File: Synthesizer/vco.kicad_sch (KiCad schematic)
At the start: 33 parts

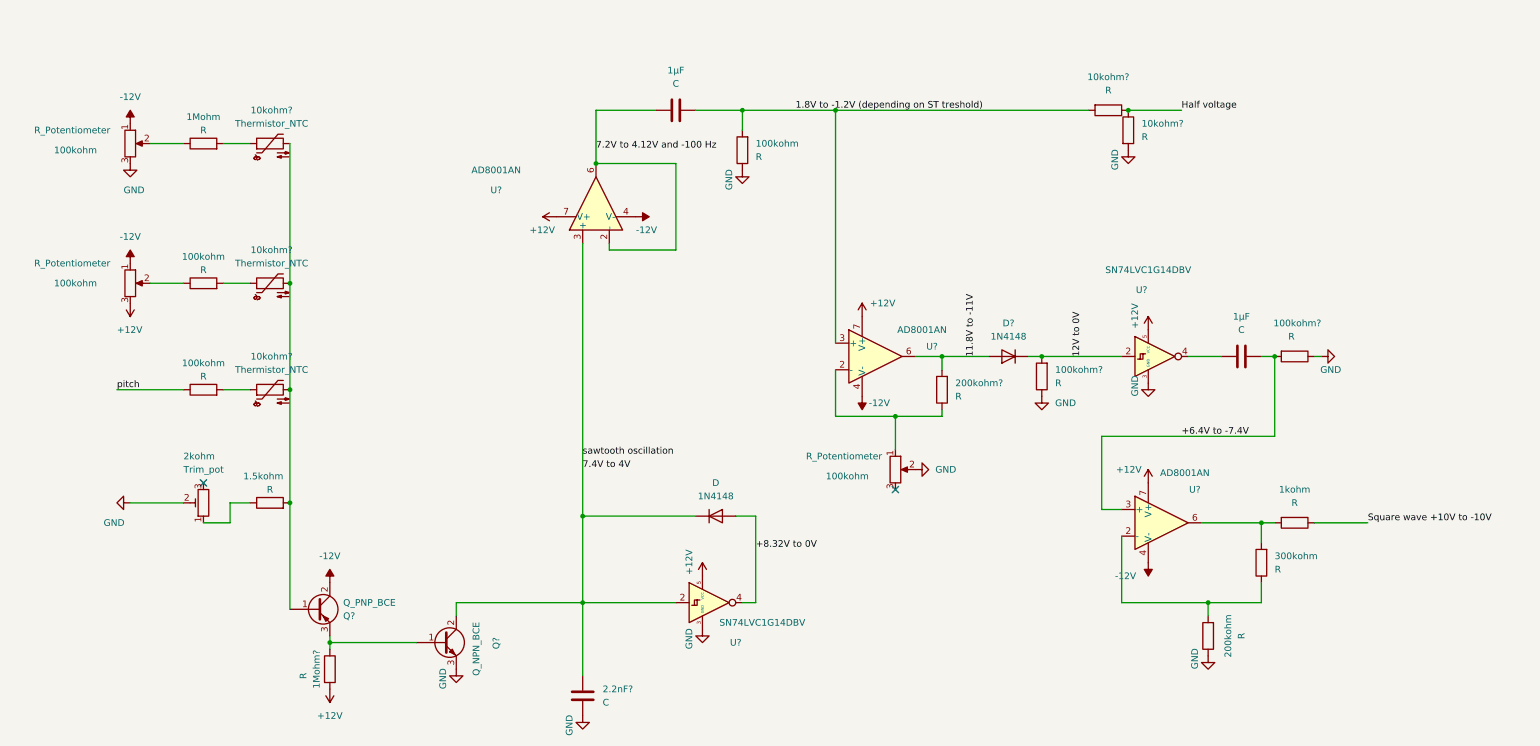
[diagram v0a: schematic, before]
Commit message: Update documentation on learnings
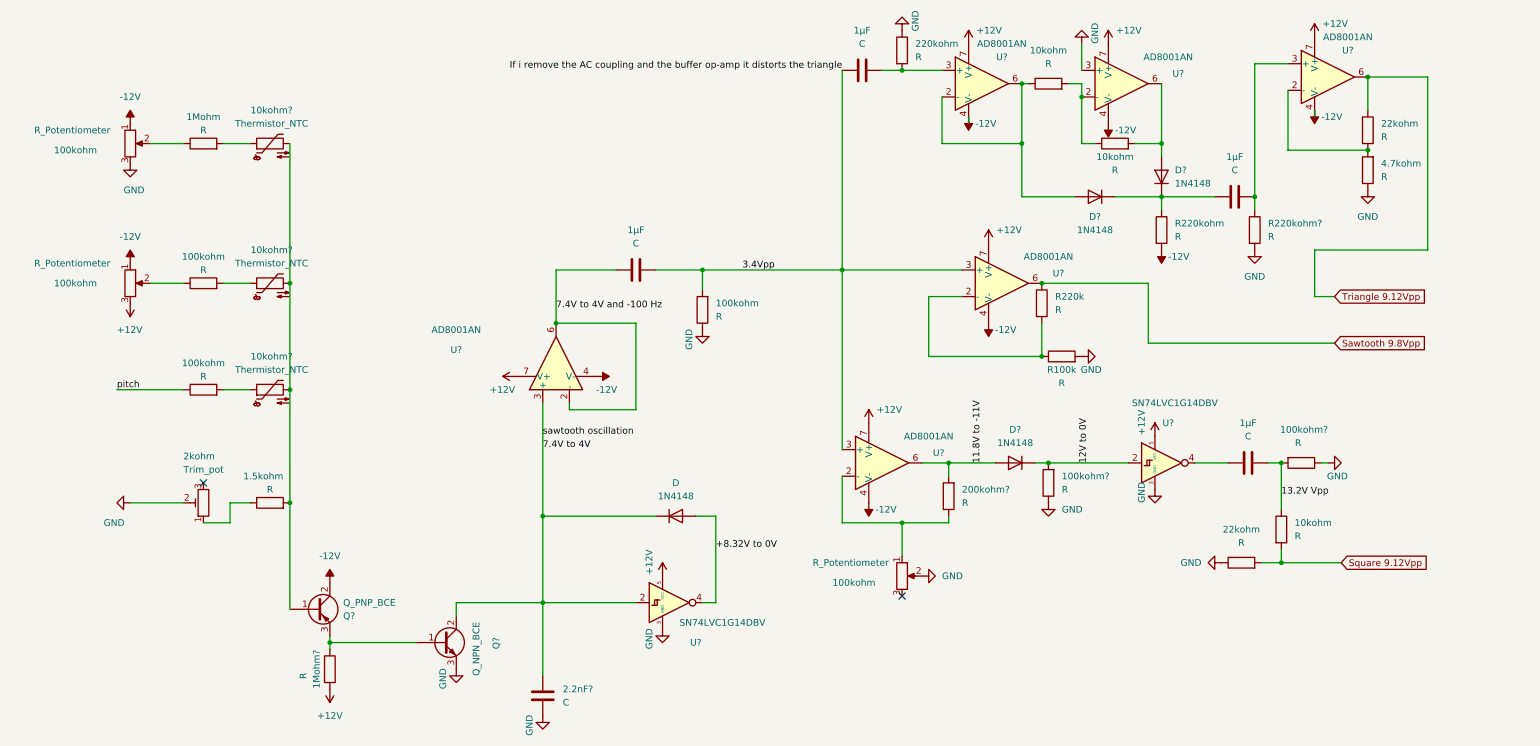
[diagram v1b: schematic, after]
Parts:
- removed 10kohm? (x2), 1kohm, 200kohm, 300kohm: R, symbol Device:R
- removed U?: AD8001AN, Package_DIP:DIP-8_W7.62mm, symbol Amplifier_Operational:AD8001AN
- added 10kohm (x3), 220kohm, 22kohm (x2), 4.7kohm, R100k, R220k, R220kohm, R220kohm?: R, symbol Device:R
- added 1µF (x2): C, symbol Device:C
- added D? (x2): 1N4148, Diode_THT:D_DO-35_SOD27_P7.62mm_Horizontal, symbol Diode:1N4148
- added U? (x4): AD8001AN, Package_DIP:DIP-8_W7.62mm, symbol Amplifier_Operational:AD8001AN
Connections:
- net +12V: now also U?.7 (V+), U?.7 (V+), U?.7 (V+), U?.7 (V+)
- net -12V: now also R220kohm.2, U?.4 (V-), U?.4 (V-), U?.4 (V-), U?.4 (V-)
- net GND: now also 220kohm.1, 22kohm.1, 4.7kohm.1, R100k.2, R220kohm?.2, U?.3 (+)
- net +6.4V to -7.4V renamed 13.2V Vpp
- net 13.2V Vpp: now also 10kohm.1
- net 1.8V to -1.2V (depending on ST treshold) renamed 3.4Vpp
- net 3.4Vpp: now also 1µF.1, U?.3 (+)
- net 7.2V to 4.12V and -100 Hz renamed 7.4V to 4V and -100 Hz
- new net: 1µF.2, 220kohm.2, U?.3 (+)
- new net: 22kohm.2, 4.7kohm.2, U?.2 (-)
- new net: 1µF.2, R220kohm?.1, U?.3 (+)
- new net: 10kohm.1, 10kohm.2, U?.2 (-)
- new net: 10kohm.2, D?.2 (A), U?.6
- new net: R100k.1, R220k.2, U?.2 (-)
- new net: 1µF.1, D?.1 (K), D?.1 (K), R220kohm.1
- new net: 10kohm.1, D?.2 (A), U?.2 (-), U?.6
- new net Sawtooth 9.8Vpp: R220k.1, U?.6
- new net Square 9.12Vpp: 10kohm.2, 22kohm.2
- new net Triangle 9.12Vpp: 22kohm.1, U?.6
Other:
- moved on the sheet: 100kohm, 100kohm?, 1µF, 2.2nF?, 200kohm?, D, D?, U?
